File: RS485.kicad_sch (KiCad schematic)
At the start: 19 parts, among them J11 430450212, J22 430450212, T1 DA2304-ALD, U4 LP2985A-50DBVR, U6 ISO3086TDW, U8 MAX485CSA_T

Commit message: assigned footprints
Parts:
- C10, C11, C19, C20, C21, C7, C9: footprint (none) -> Capacitor_SMD:C_0805_2012Metric
- J11, J22: footprint CON_430450212_MOL -> RS485-Header:CON_430450212_MOL
- R30, R39, R44, R45: footprint (none) -> Resistor_SMD:R_0805_2012Metric
- U4: footprint LP2985A-50DBVR:SOT95P280X145-5N -> LP2985A_50DBVR:SOT95P280X145-5N
- U6: footprint DW16 -> ISO3086TDW:DW16
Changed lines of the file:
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@@
 			)
 		)
-		(property "Footprint" "CON_430450212_MOL"
+		(property "Footprint" "RS485-Header:CON_430450212_MOL"
 			(at 259.08 41.91 0)
 			(effects
@@
 			)
 		)
-		(property "Footprint" ""
+		(property "Footprint" "Capacitor_SMD:C_0805_2012Metric"
 			(at 89.8652 110.49 0)
 			(effects
@@
 			)
 		)
-		(property "Footprint" ""
+		(property "Footprint" "Resistor_SMD:R_0805_2012Metric"
 			(at 215.9 98.298 90)
 			(effects
@@
 			)
 		)
-		(property "Footprint" ""
+		(property "Footprint" "Resistor_SMD:R_0805_2012Metric"
 			(at 214.63 118.618 90)
 			(effects
@@
 			)
 		)
-		(property "Footprint" ""
+		(property "Footprint" "Resistor_SMD:R_0805_2012Metric"
 			(at 215.9 94.488 90)
 			(effects
@@
 			)
 		)
-		(property "Footprint" ""
+		(property "Footprint" "Resistor_SMD:R_0805_2012Metric"
 			(at 214.63 122.428 90)
 			(effects
@@
 			)
 		)
-		(property "Footprint" "DW16"
+		(property "Footprint" "ISO3086TDW:DW16"
 			(at 138.43 43.18 0)
 			(effects
@@
 			)
 		)
-		(property "Footprint" ""
+		(property "Footprint" "Capacitor_SMD:C_0805_2012Metric"
 			(at 204.1652 43.18 0)
 			(effects
@@
 			)
 		)
-		(property "Footprint" ""
+		(property "Footprint" "Capacitor_SMD:C_0805_2012Metric"
 			(at 41.91 108.2548 0)
 			(effects
@@
 			)
 		)
-		(property "Footprint" ""
+		(property "Footprint" "Capacitor_SMD:C_0805_2012Metric"
 			(at 214.3252 43.18 0)
 			(effects
@@
 			)
 		)
-		(property "Footprint" "CON_430450212_MOL"
+		(property "Footprint" "RS485-Header:CON_430450212_MOL"
 			(at 259.08 58.42 0)
 			(effects
@@
 			)
 		)
-		(property "Footprint" "LP2985A-50DBVR:SOT95P280X145-5N"
+		(property "Footprint" "LP2985A_50DBVR:SOT95P280X145-5N"
 			(at 149.86 110.49 0)
 			(effects
@@
 			)
 		)
-		(property "Footprint" ""
+		(property "Footprint" "Capacitor_SMD:C_0805_2012Metric"
 			(at 129.2352 119.38 0)
 			(effects
@@
 			)
 		)
-		(property "Footprint" ""
+		(property "Footprint" "Capacitor_SMD:C_0805_2012Metric"
 			(at 79.7052 110.49 0)
 			(effects
@@
 			)
 		)
-		(property "Footprint" ""
+		(property "Footprint" "Capacitor_SMD:C_0805_2012Metric"
 			(at 93.6752 44.45 0)
 			(effects

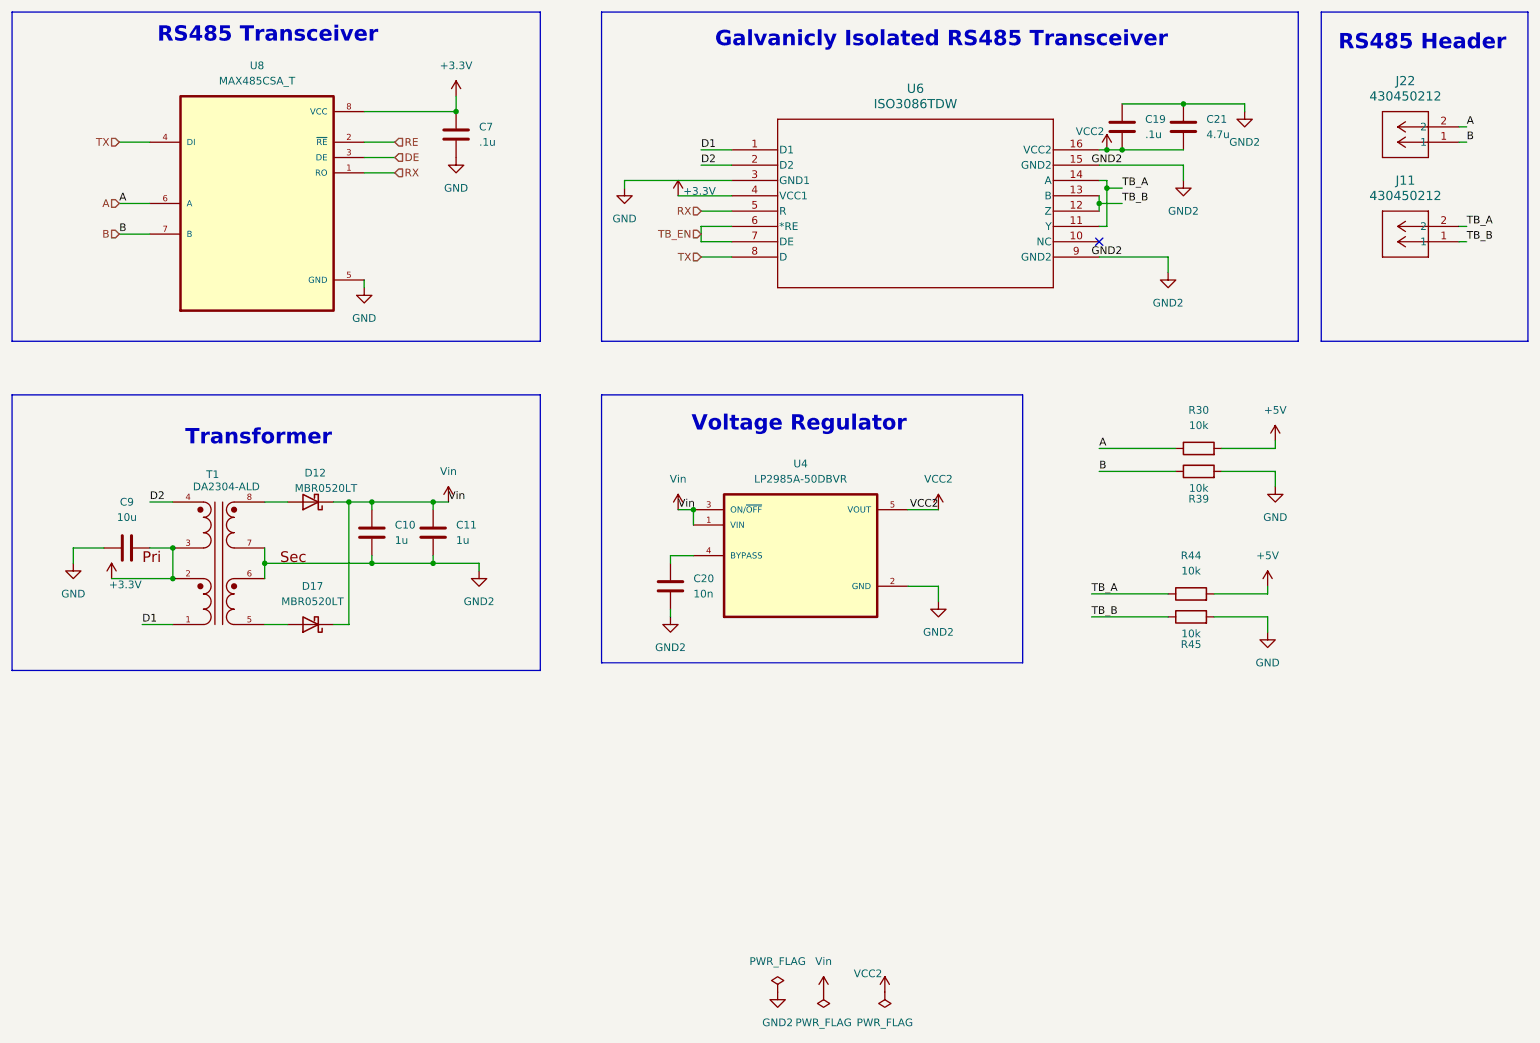
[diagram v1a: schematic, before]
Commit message: stuff
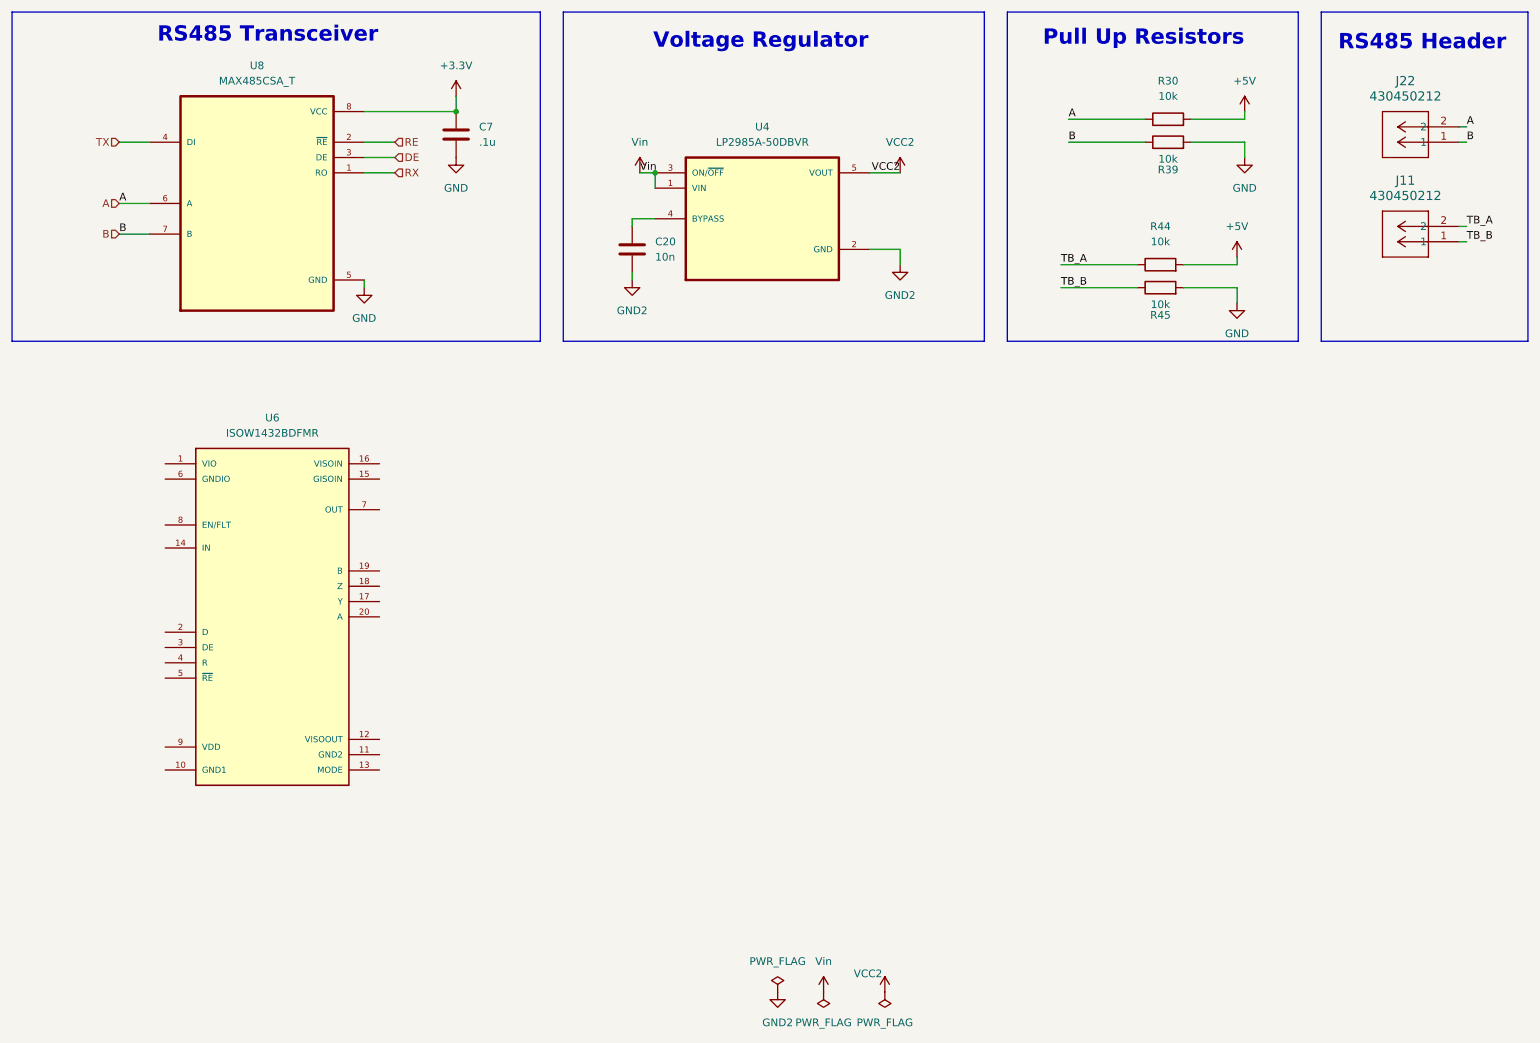
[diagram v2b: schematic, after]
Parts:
- removed C10, C11: 1u, Capacitor_SMD:C_0805_2012Metric, symbol Device:C
- removed C19: .1u, Capacitor_SMD:C_0805_2012Metric, symbol Device:C
- removed C21: 4.7u, Capacitor_SMD:C_0805_2012Metric, symbol Device:C
- removed C9: 10u, Capacitor_SMD:C_0805_2012Metric, symbol Device:C
- removed D12, D17: MBR0520LT, Diode_SMD:D_SOD-123, symbol Diode:MBR0520LT
- removed T1: DA2304-ALD, DA2304-ALD:XFMR_DA2304-ALD, symbol DA2304-ALD:DA2304-ALD
- removed U6: ISO3086TDW, ISO3086TDW:DW16, symbol ISO3086T:ISO3086TDW
- added U6: ISOW1432BDFMR, ISOW1432BDFMR:SOIC127P1030X355-20N, symbol ISOW1432BDFMR:ISOW1432BDFMR
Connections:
- no-connect marks 1 -> 0
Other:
- note added: "Pull Up Resistors"
- note removed: "Galvanicly Isolated RS485 Transceiver"
- note removed: "Transformer"
- moved on the sheet: C20, R30, R39, R44, R45, U4
